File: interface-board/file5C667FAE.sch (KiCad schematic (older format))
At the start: 27 parts, among them U4 LTV-817S, U5 DCM4623TD2J13D0T70, U6 LTV-817S, U7 R-78E5.0-0.5, U9 TLP184

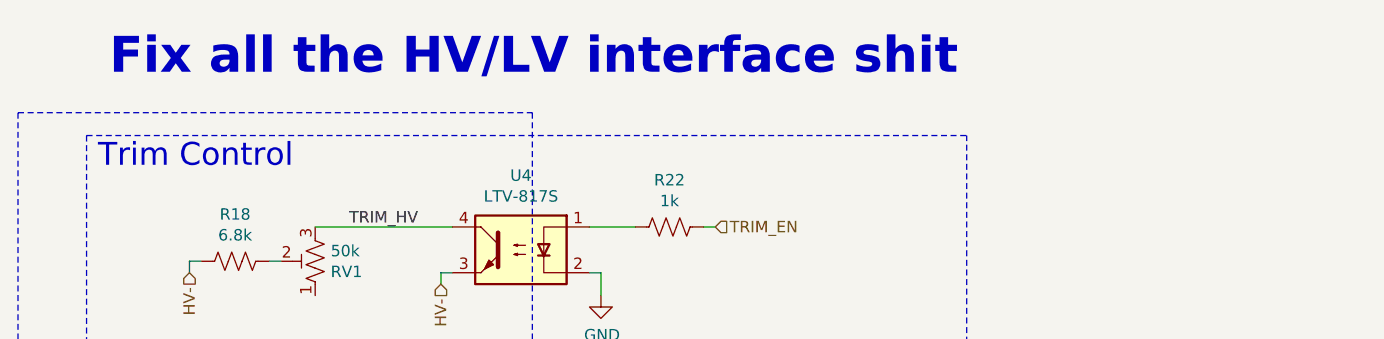
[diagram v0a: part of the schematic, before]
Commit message: Cleaned up 3d models
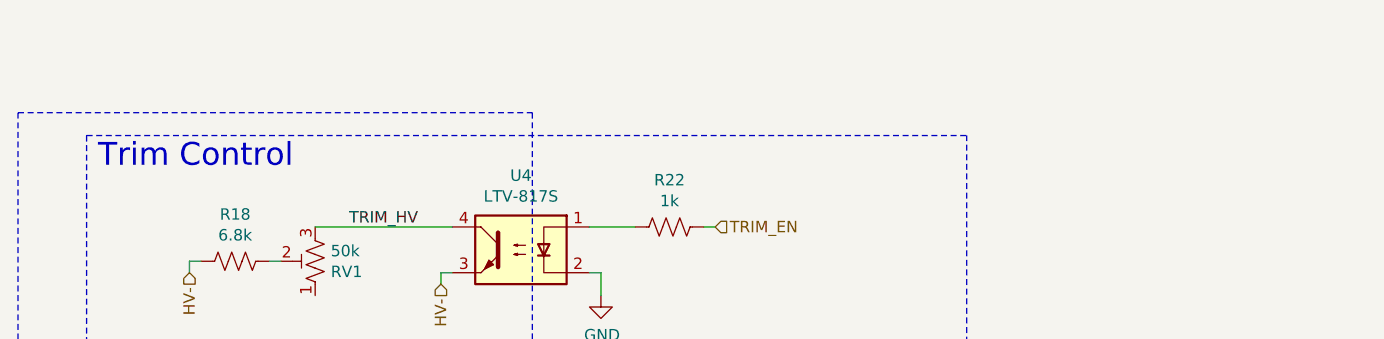
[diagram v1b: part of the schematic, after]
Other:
- note removed: "Fix all the HV/LV interface shit"
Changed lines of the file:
@@
 Wire Notes Line width 39 rgb(255, 0, 0)
 	3150 1150 3150 6300
-Text Notes 3550 1000 0    157  ~ 31
-Fix all the HV/LV interface shit
 $Comp
 L Device:R_US R18
